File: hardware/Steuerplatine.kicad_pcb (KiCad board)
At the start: 2 copper layers, 110 x 110 mm, 62 parts, among them J1 Conn_01x02_Pin, J2 Conn_01x02_Pin, Q1 BC848, Q2 BTA16-600B, Q3 BC848, U1 LPS28DFW, U2 LNK3202D, U4 TL082, U5 Seeed-ESP32C3

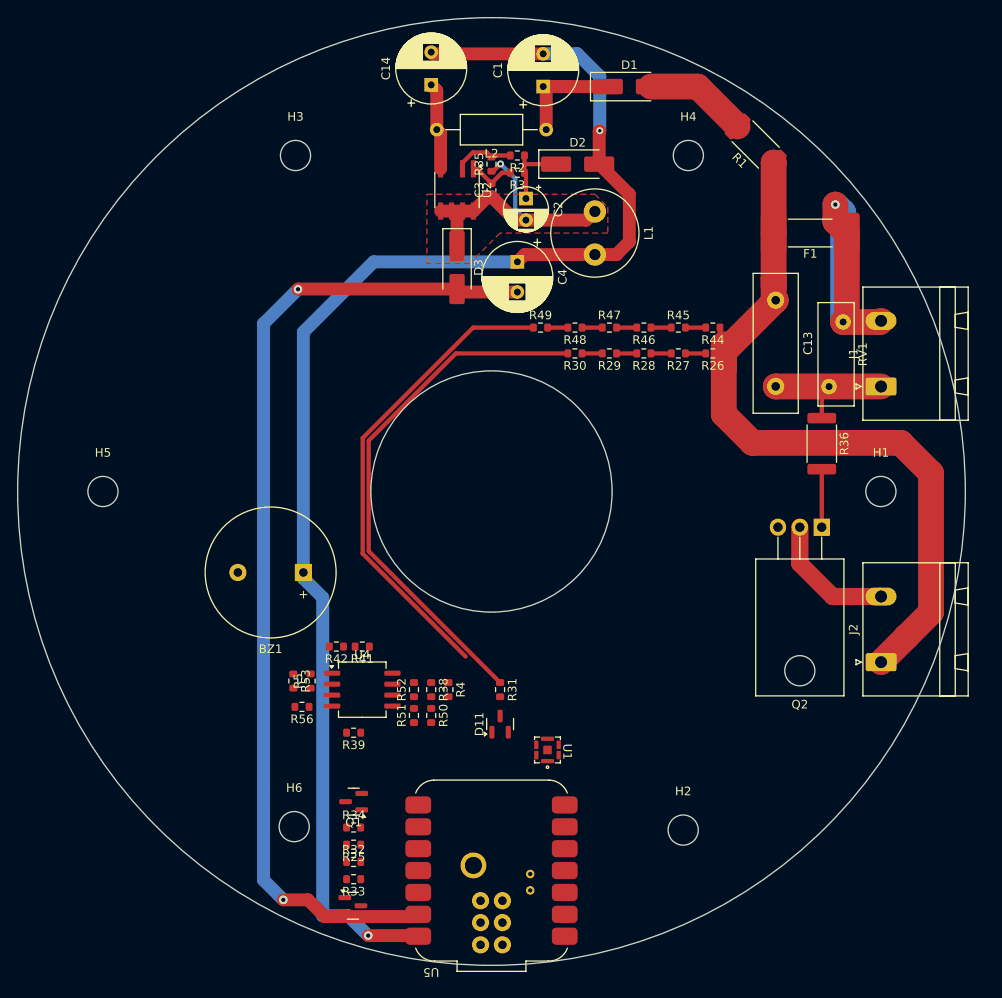
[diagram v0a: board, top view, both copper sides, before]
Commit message: added some zones
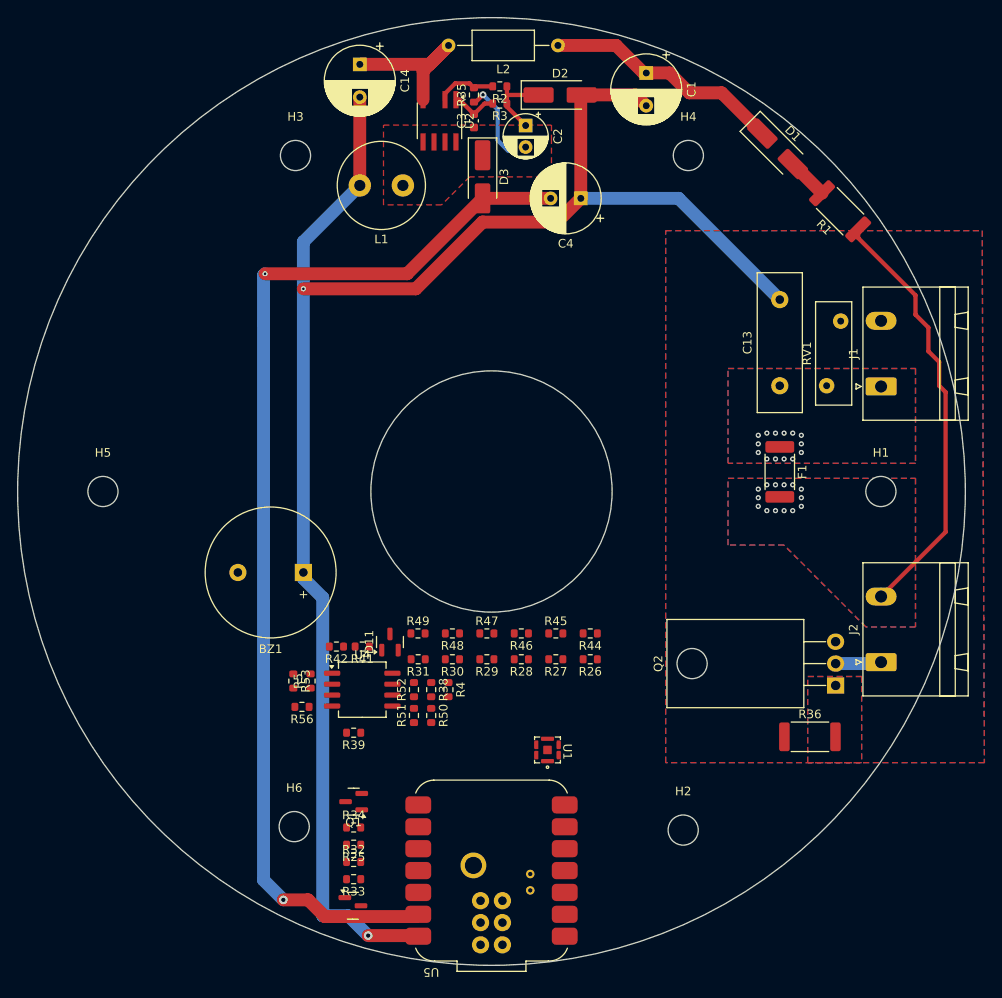
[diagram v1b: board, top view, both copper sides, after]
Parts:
- F1: footprint Fuse:Fuse_Schurter_UMZ250 -> Fuse:Fuse_2512_6332Metric
- moved R26 38.2 mm to (165.2, 160.5)
- moved R27 38.2 mm to (161.2, 160.5)
- moved R28 38.2 mm to (157.2, 160.5)
- moved R29 38.2 mm to (153.2, 160.5)
- moved R30 38.2 mm to (149.2, 160.5)
- moved R44 38.2 mm to (165.2, 157.5)
- moved R45 38.2 mm to (161.2, 157.5)
- moved R46 38.2 mm to (157.2, 157.5)
- moved R47 38.2 mm to (153.2, 157.5)
- moved R48 38.2 mm to (149.2, 157.5)
- moved R49 38.2 mm to (145.2, 157.5)
- moved R36 34.1 mm to (190.8, 169.5), turned to 0 degrees
- moved F1 27.9 mm to (187.2, 138.8), turned to -90 degrees
- moved L1 22.5 mm to (143.5, 105.5), turned to 180 degrees
- moved D1 18.7 mm to (187.0, 101.2), turned to -45 degrees
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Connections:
- C13 pad 1: /L_filt -> /L
- J1 pad 1: /+5V -> /L
- J1 pad 2: /L -> /+5V
- J2 pad 1: /L_filt -> /Triac/TRIAC_OUTPUT
- J2 pad 2: /Triac/TRIAC_OUTPUT -> /L_filt
- U1 pad 4: unconnected-(U1-INT_DRDY-Pad4) -> /Controller/pressure_interrupt
- U1 pad 7: unconnected-(U1-PAD2LID-Pad7) -> /GND
- U5 pad 7: unconnected-(U5-D6-Pad7) -> /Controller/pressure_interrupt
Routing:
- net Net-(R30-Pad2): track 61.7 -> 0.00 mm
- net Net-(R49-Pad1): track 55.4 -> 0.00 mm
- net /L_filt: track 90.0 -> 49.9 mm, vias 0 -> 14
- net /L: track 32.8 -> 0.00 mm, vias 1 -> 14
- net Net-(D3-K): track 33.6 -> 9.15 mm
- net /+5V: track 180.6 -> 195.3 mm
- net Net-(D1-K): track 15.4 -> 28.0 mm
- net /GND: track 115.7 -> 127.0 mm
- net /Triac/TRIAC_OUTPUT: track 15.3 -> 5.36 mm
- net Net-(U2-D): track 10.2 -> 18.7 mm
- net Net-(D1-A): track 12.0 -> 4.79 mm
- net Net-(Q2-A1): track 6.74 -> 0.00 mm
- net Net-(R48-Pad2): track 2.35 -> 0.00 mm
- net Net-(R47-Pad1): track 2.35 -> 0.00 mm
- net Net-(R46-Pad2): track 2.35 -> 0.00 mm
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- added copper zone on B.Cu, net /+5V
- added copper zone on F.Cu, net /+5V
- added copper zone on B.Cu, net /L
- added copper zone on F.Cu, net /L
- added copper zone on B.Cu, net /L_filt
- added copper zone on F.Cu, net /L_filt
- added copper zone on B.Cu, net Net-(Q2-A1)
- added copper zone on F.Cu, net Net-(Q2-A1)
